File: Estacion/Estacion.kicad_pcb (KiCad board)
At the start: 2 copper layers, 120 x 64.1 mm, 12 parts, among them SW1 SW_Push, U4 WeMos_S2_mini, U5 DHT22, U6 FN-M16P

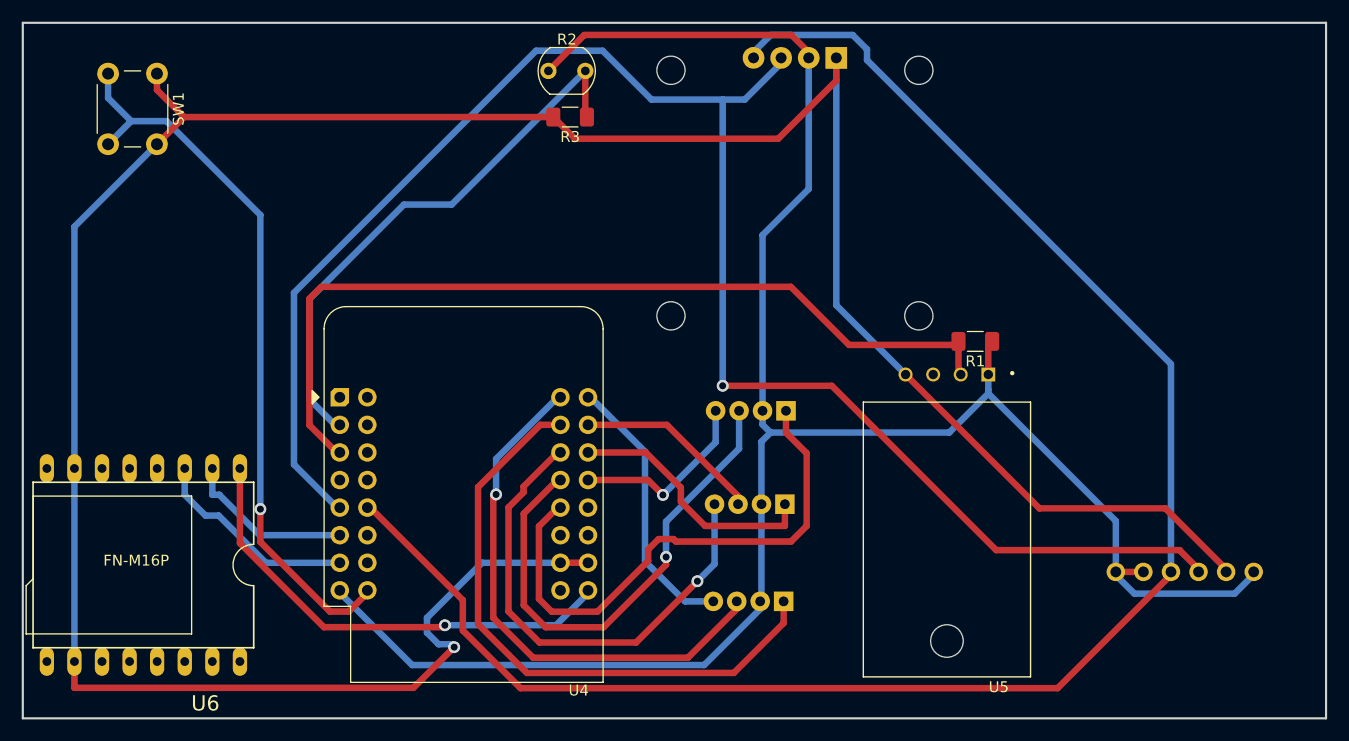
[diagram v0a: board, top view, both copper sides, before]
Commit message: Hola pipol de youtube
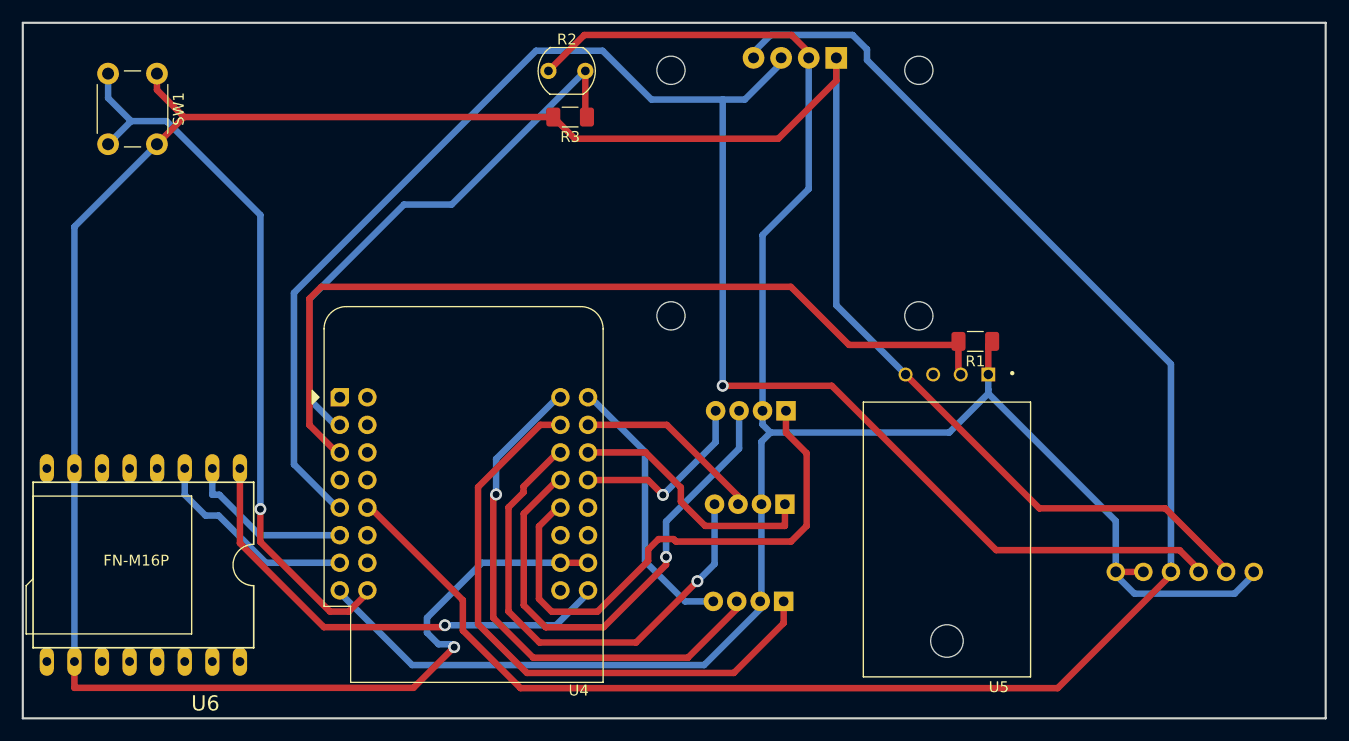
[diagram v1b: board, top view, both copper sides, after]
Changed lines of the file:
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@@
 		(capping no)
 		(filling no)
-		(zone_defaults)
 		(pcbplotparams
 			(layerselection 0x00000000_00000000_55555555_5755f5ff)
@@
 	(gr_rect
 		(start 64.897 52.07)
-		(end 184.912 116.12)
+		(end 184.88 116.12)
 		(stroke
 			(width 0.2)
